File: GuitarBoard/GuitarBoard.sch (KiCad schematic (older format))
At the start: 49 parts, among them IC1 CD4069UBE, J1 Pickups, J2 Input Jack, J3 Bridge Ground, J8 Output Jack, J9 Amp, Q1 2N3904, Q2 2N3904, SW1 Amp Knob Switch, SW2 Volume DPDT A, SW3 Volume DPDT B, SW4 Tone DPDT A, SW5 Tone DPDT B

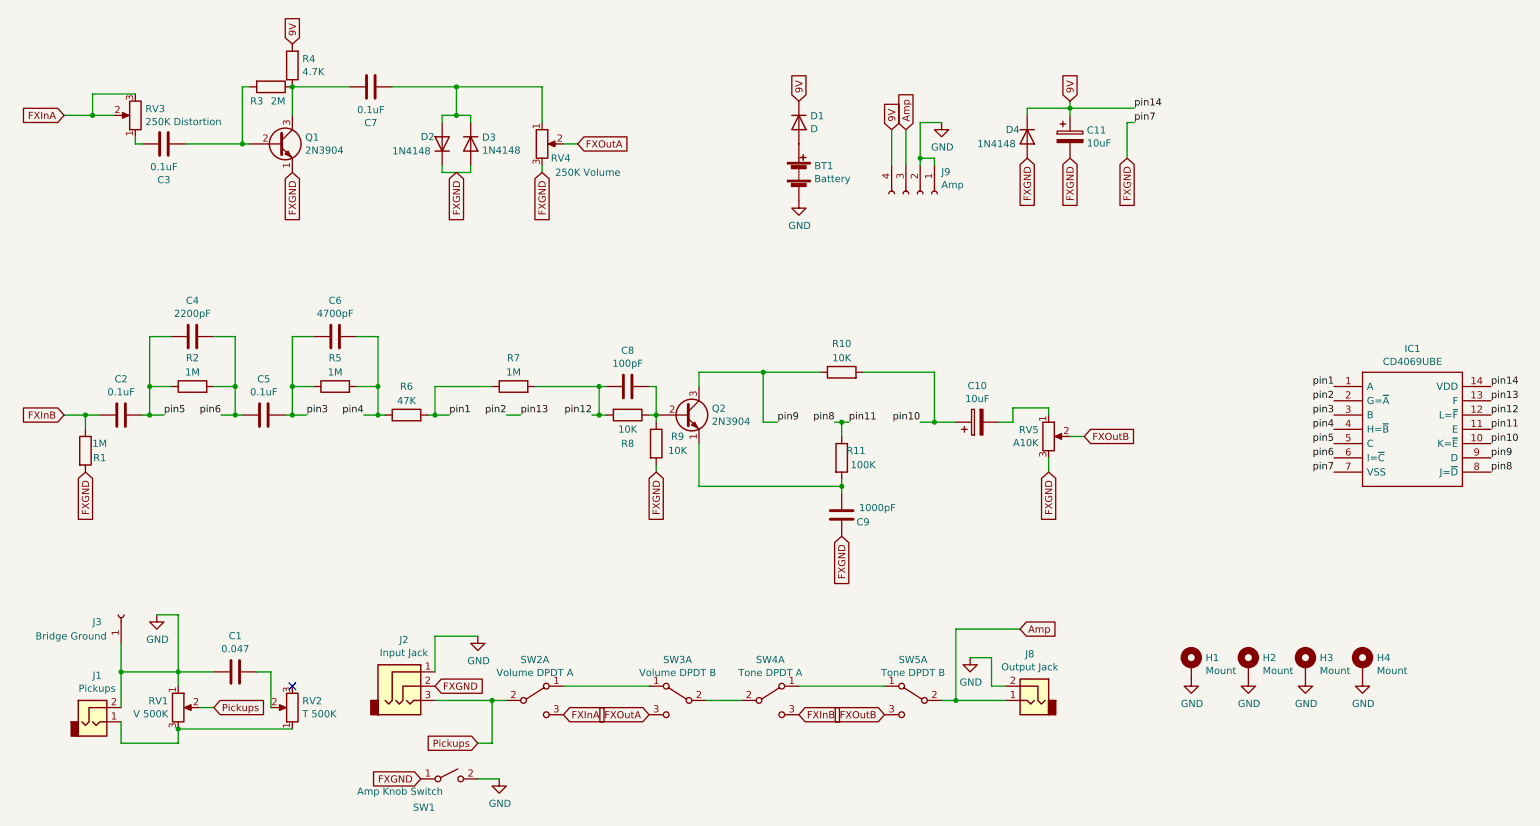
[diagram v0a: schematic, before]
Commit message: Made new board. Still need to lay out all the traces
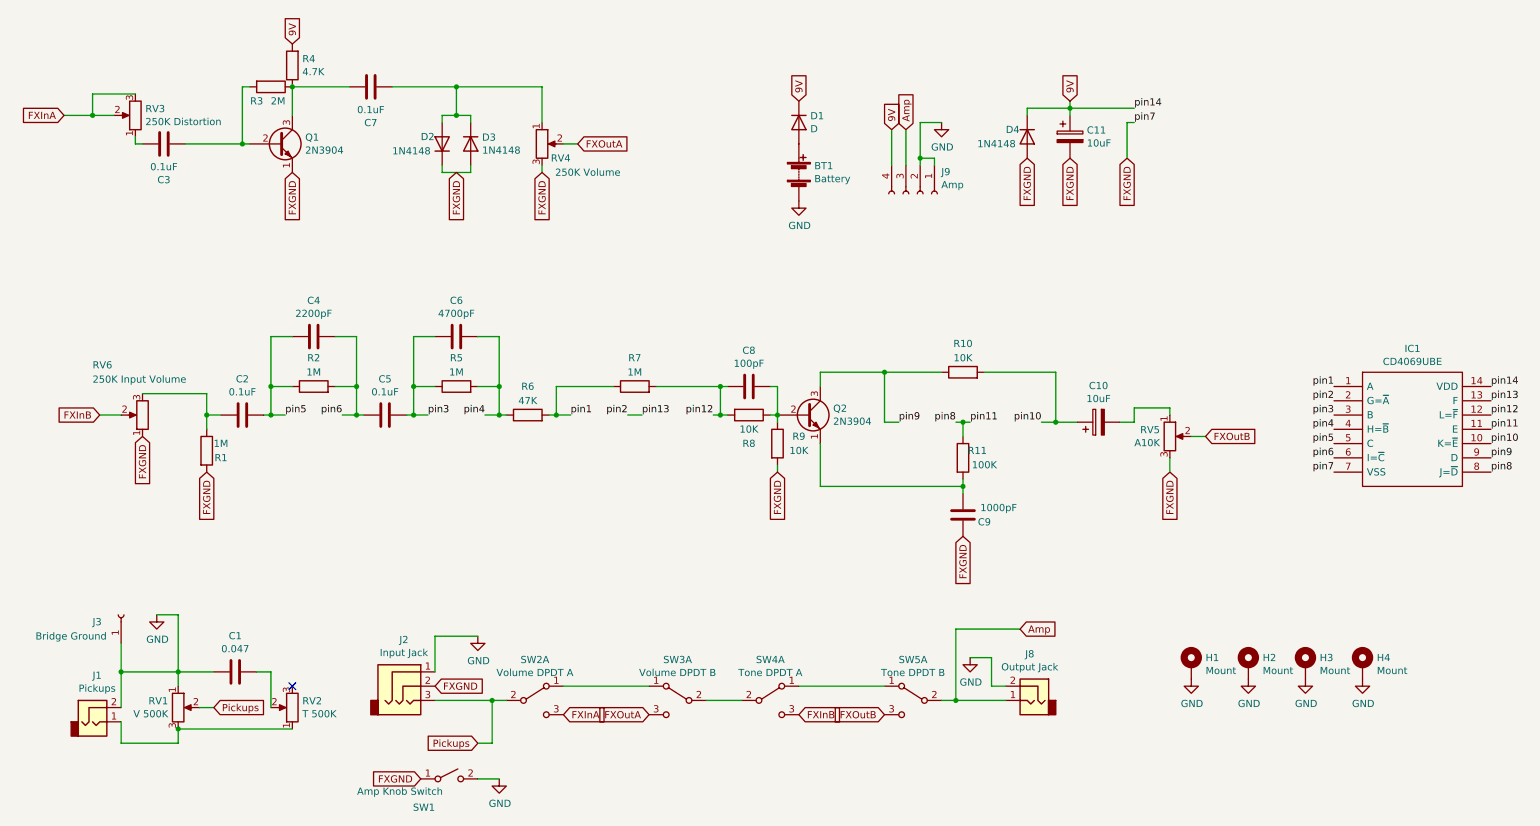
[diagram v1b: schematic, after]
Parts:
- added RV6: 250K Input Volume, Potentiometer_THT:Potentiometer_Bourns_3386F_Vertical, symbol Device:R_POT
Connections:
- net FXGND: now also RV6.1
- net FXInB: now also RV6.2; no longer C2.2, R1.1
- new net: C2.2, R1.1, RV6.3
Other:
- moved on the sheet: C10, C2, C4, C5, C6, C8, C9, Q2, R1, R10, R11, R2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
